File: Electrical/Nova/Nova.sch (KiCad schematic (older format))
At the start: 0 parts

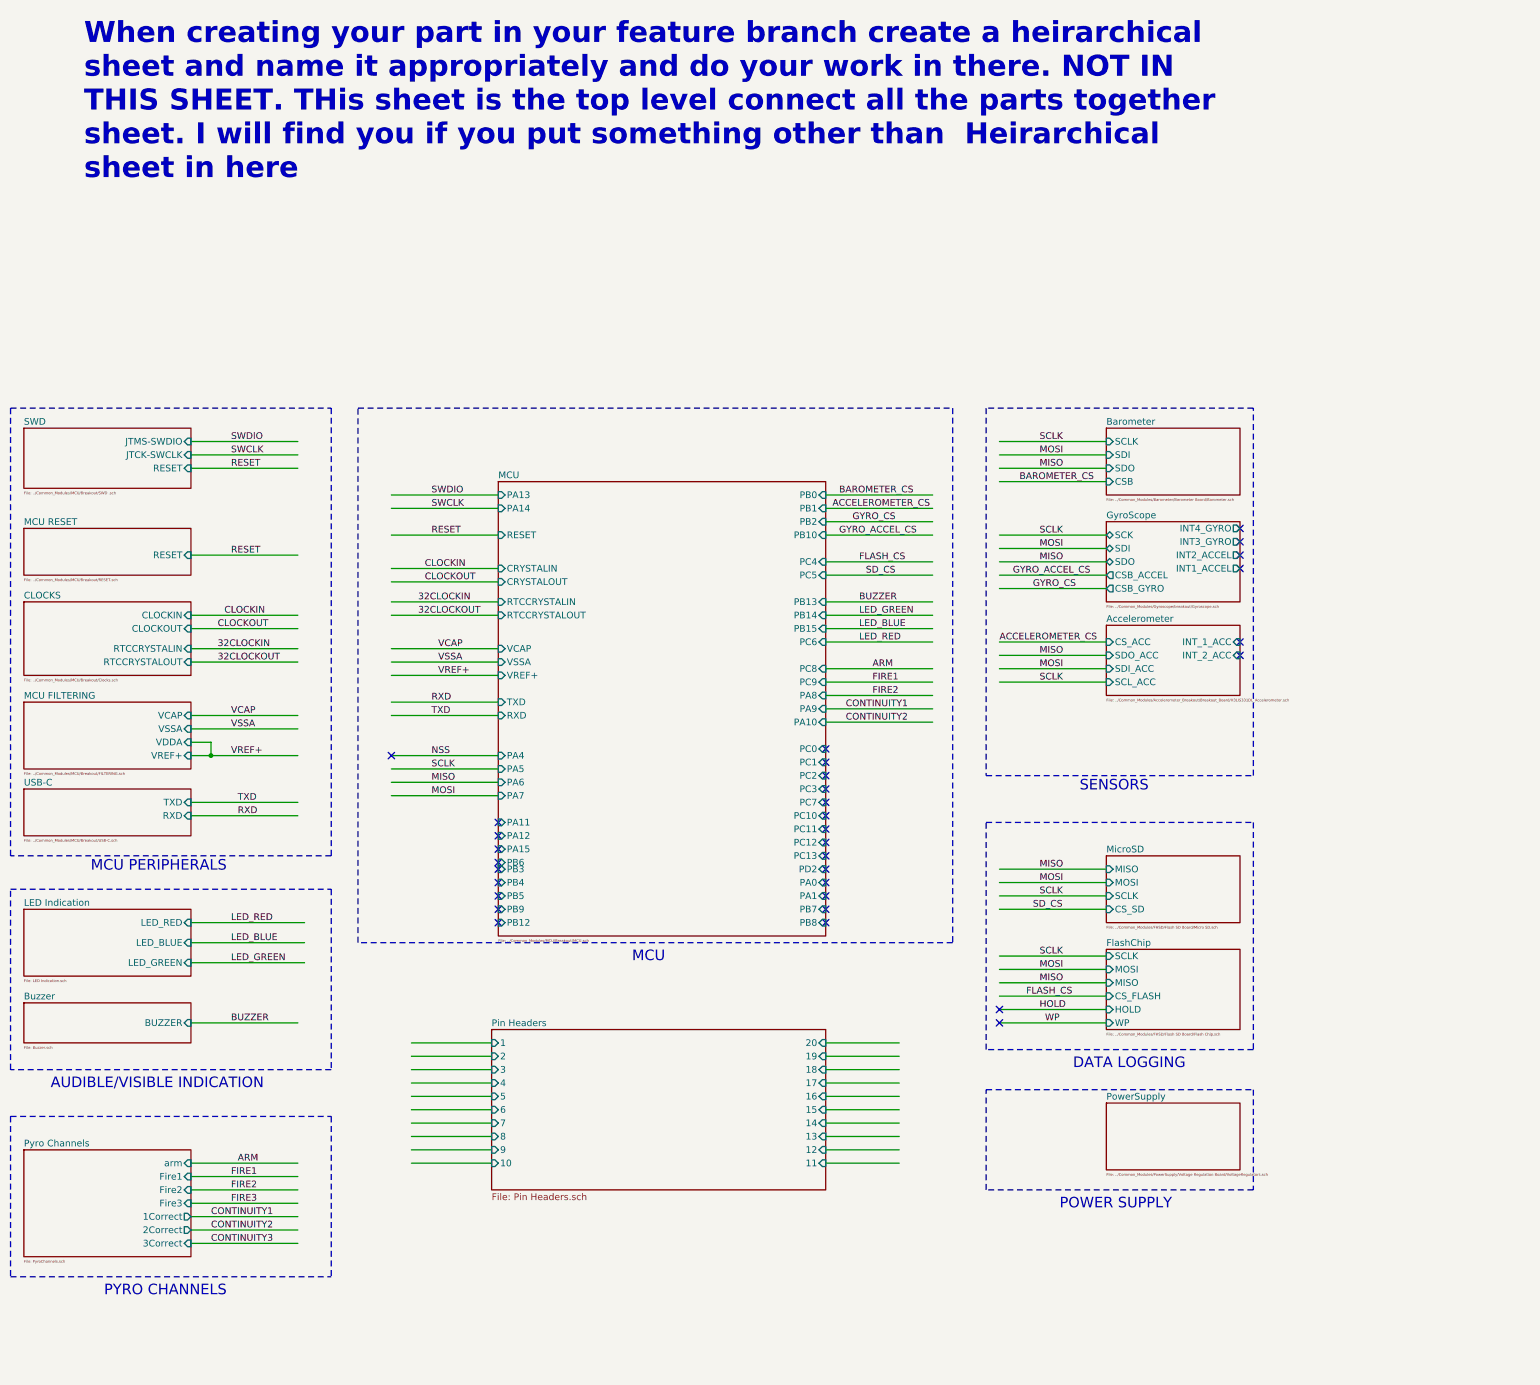
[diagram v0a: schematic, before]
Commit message: Cleaned Up Schematic & Folder for Project
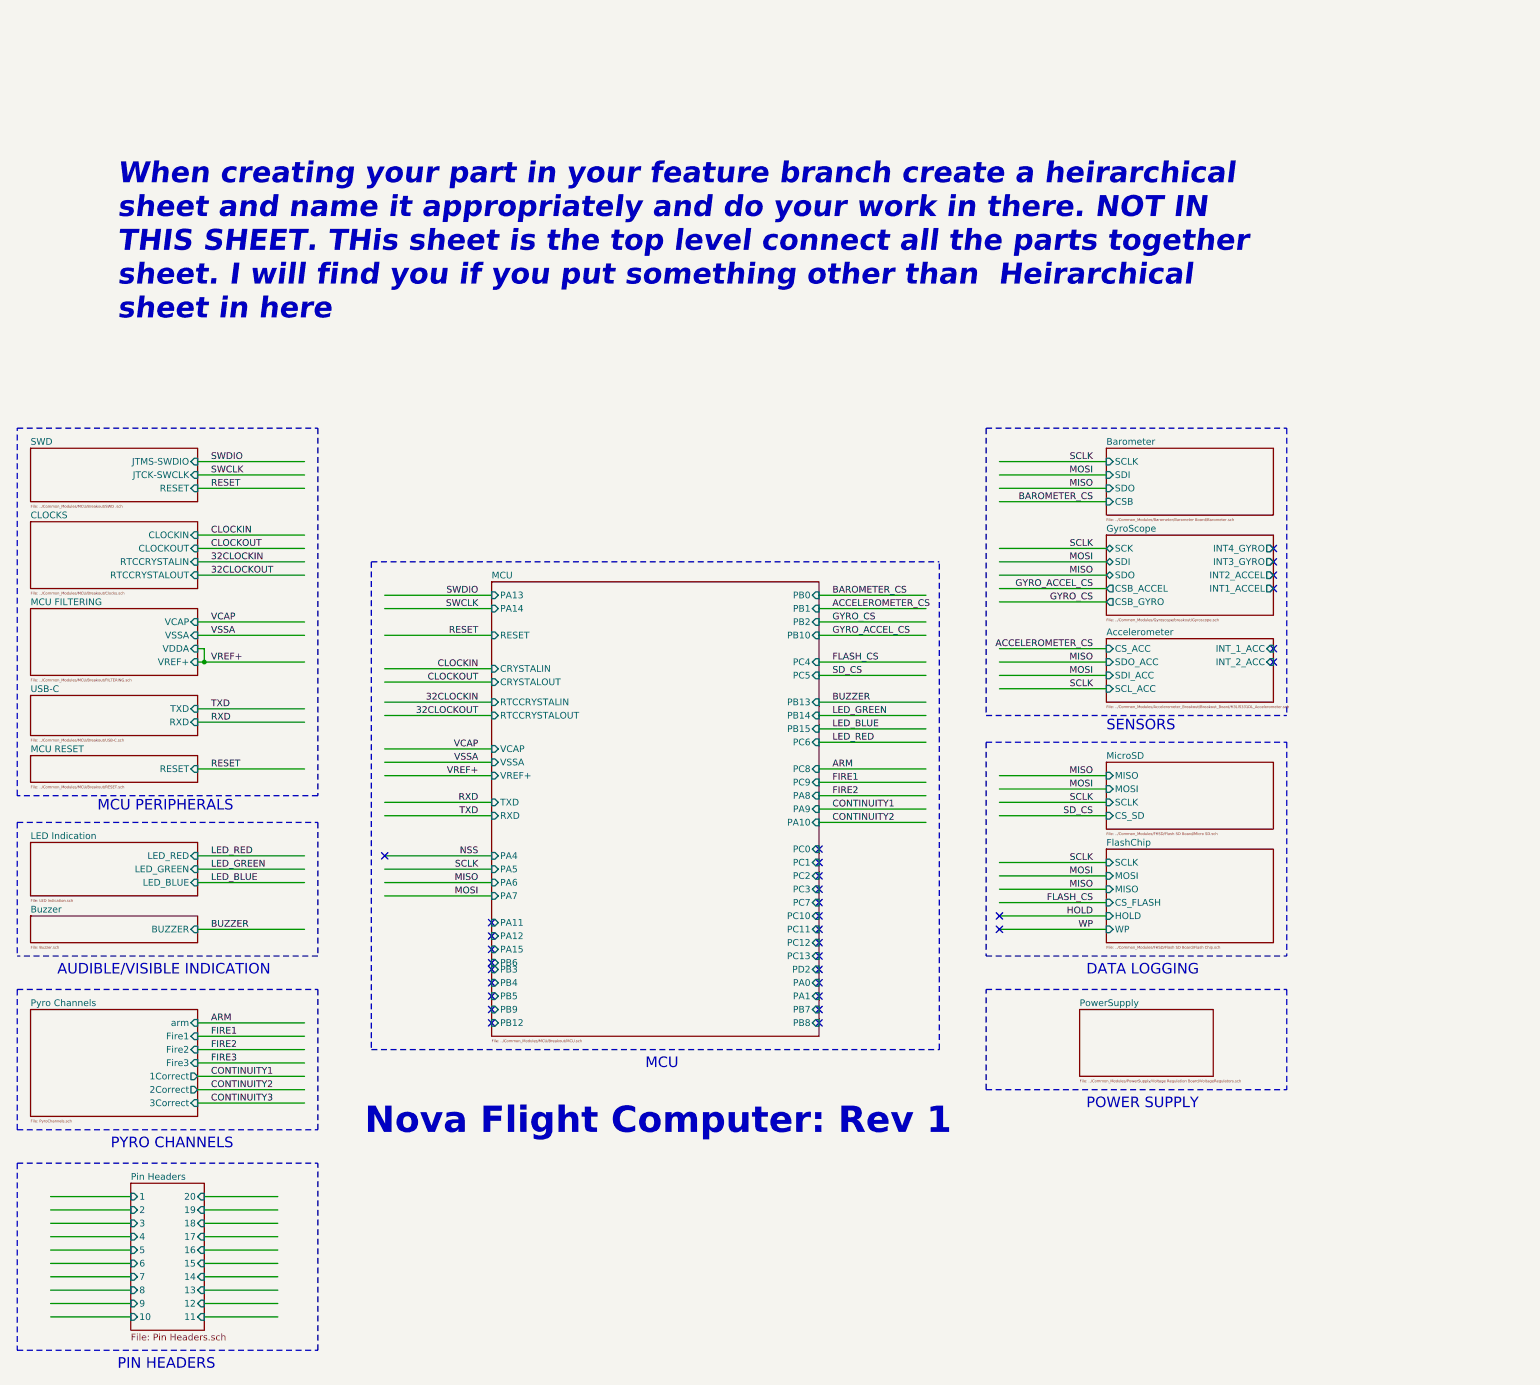
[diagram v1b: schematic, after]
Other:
- note added: "Nova Flight Computer: Rev 1"
- note added: "PIN HEADERS"
